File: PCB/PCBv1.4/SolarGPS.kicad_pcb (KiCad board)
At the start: 2 copper layers, 78 x 32 mm, 43 parts, among them J1 Conn_01x24_Female, J2 GND, J3 GND, J4 Conn_02x03_Odd_Even, J5 Solar2+, J6 Solar1+, J7 Screw_Terminal_01x01, J8 Conn_01x04_Male, Q1 Q_NMOS_GSD, U1 STM32L011G4Ux, U2 MAX-M10Q, U6 LIS3DH, Y1 32.768

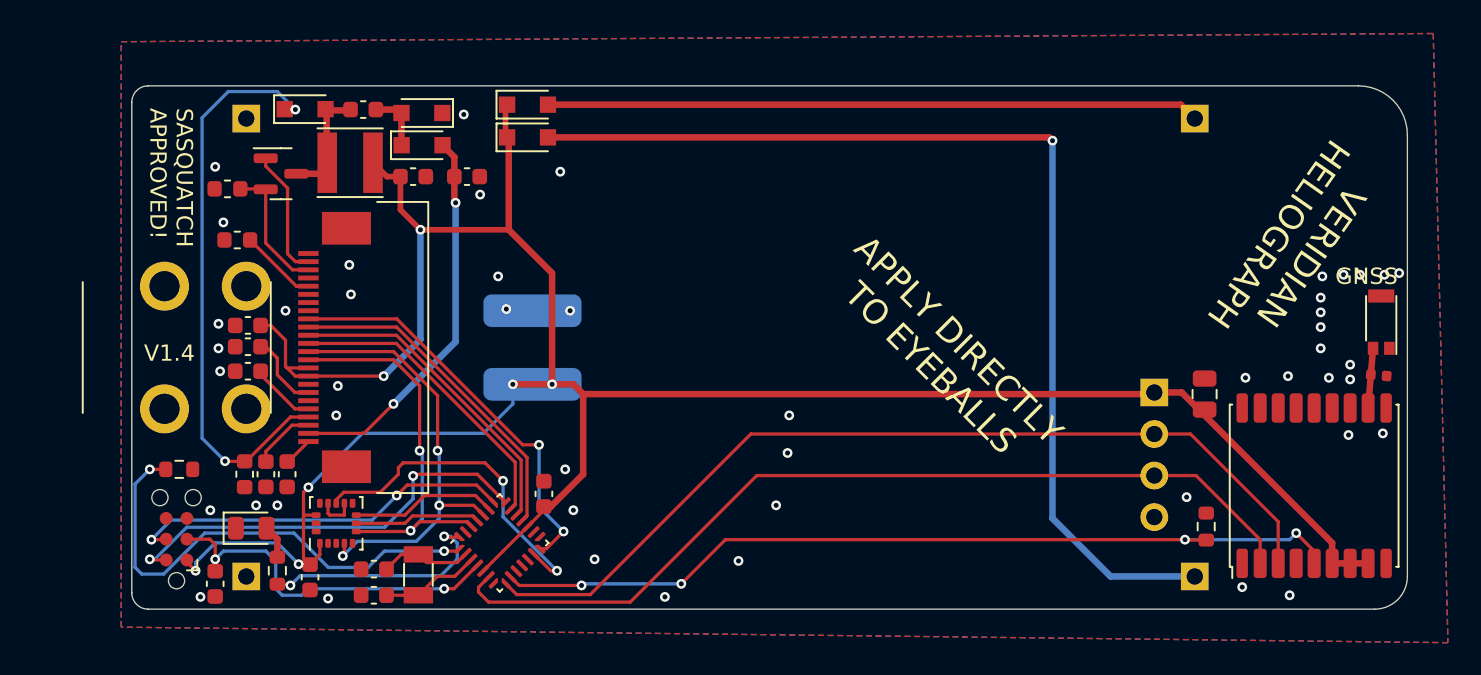
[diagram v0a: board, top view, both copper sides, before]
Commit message: firmware stuff
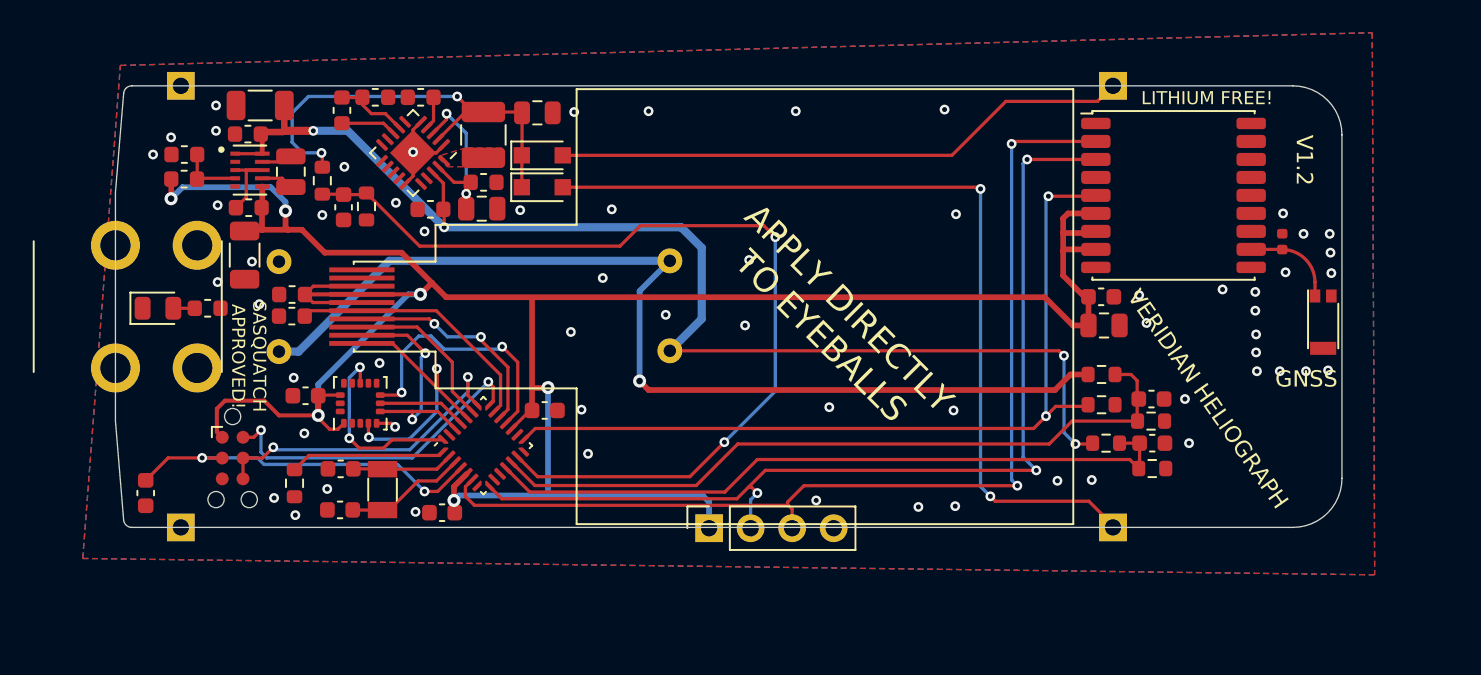
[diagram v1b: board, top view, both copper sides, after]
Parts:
- removed C22: 1uF, Capacitor_SMD:C_0603_1608Metric
- removed D4, D5, D6: B0530WS, Diode_SMD:D_SOD-323_HandSoldering
- removed L1: 47uH, Inductor_SMD:L_Taiyo-Yuden_NR-40xx
- removed Q1: Q_NMOS_GSD, Package_TO_SOT_SMD:SOT-23
- added C11: 1uF, Capacitor_SMD:C_0603_1608Metric, F.Cu at (75.2, 69.8)
- added C12: 47uF, Capacitor_SMD:C_1206_3216Metric, F.Cu at (57.9, 51.2)
- added C13: 4.7uF, Capacitor_SMD:C_0805_2012Metric, F.Cu at (109.5, 64.7)
- added C14: 10F, Veridian-Library-KiCad:SCCT20E106SRB, B.Cu at (82.9, 63.5)
- added C17: 10F, Veridian-Library-KiCad:SCCT20E106SRB, B.Cu at (59.0, 63.5)
- added C19: 10nF, Capacitor_SMD:C_0603_1608Metric, F.Cu at (71.5, 55.9)
- added C23: 10nF, Capacitor_SMD:C_0603_1608Metric, F.Cu at (112.4, 71.8)
- added C28: 10nF, Capacitor_SMD:C_0603_1608Metric, F.Cu at (63.0, 57.4)
- added L2: 0.47uH, Inductor_SMD:L_0806_2016Metric, F.Cu at (59.7, 55.2)
- added L3: 22uH, Inductor_SMD:L_1210_3225Metric, F.Cu at (71.5, 53.0)
- added R12: 1M, Resistor_SMD:R_0603_1608Metric, F.Cu at (109.6, 71.8)
- added R13: 1M, Resistor_SMD:R_0603_1608Metric, F.Cu at (112.4, 73.4)
- added R14: 1M, Resistor_SMD:R_0603_1608Metric, F.Cu at (61.6, 55.8)
- added R15: 1M, Resistor_SMD:R_0603_1608Metric, F.Cu at (64.3, 57.4)
- added R4: 432k, Resistor_SMD:R_0603_1608Metric, F.Cu at (53.2, 55.7)
- added R5: 91k, Resistor_SMD:R_0603_1608Metric, F.Cu at (53.2, 54.2)
- added R6: 1M, Resistor_SMD:R_0603_1608Metric, F.Cu at (112.3, 70.5)
- added ROV3: 4.30M, Resistor_SMD:R_0603_1608Metric, F.Cu at (64.9, 50.7)
- added ROV4: 8.66M, Resistor_SMD:R_0603_1608Metric, F.Cu at (62.9, 51.5)
- added U5: BQ25505, Package_DFN_QFN:QFN-20-1EP_3.5x3.5mm_P0.5mm_EP2x2mm, F.Cu at (67.2, 54.1)
- added U7: TPS63802, Margo_Lib:VREG_TPS63802DLAR, F.Cu at (57.2, 55.1)
- C15, C16, C18, C6: value 1uF -> 10nF
- C2, C3: value 1uF -> 4.7uF; footprint Capacitor_SMD:C_0603_1608Metric -> Capacitor_SMD:C_0805_2012Metric
- C5: value 22uF -> 10nF; footprint Capacitor_SMD:C_0805_2012Metric -> Capacitor_SMD:C_0603_1608Metric
- C7: value 1uF -> 47uF; footprint Capacitor_SMD:C_0603_1608Metric -> Capacitor_SMD:C_1206_3216Metric
- C8: value 25F -> 1uF; footprint Heliograph:TPLC3R8-25MR8X20 -> Capacitor_SMD:C_0603_1608Metric; moved to F.Cu
- D1, D3: value B0530WS -> Schottky
- J1: value Conn_01x24_Female -> Conn_01x10_Female; footprint Heliograph:ER-CON24HT-1 -> Margo_Lib:LS013B7DH03
- J2: value GND -> Solar1+
- J6: value Solar1+ -> GND
- J8: moved to F.Cu
- R1: value 1M -> 91k
- R2: value 120 -> 1M
- R3: value 2.2 -> 390
- U1: value STM32L011G4Ux -> STM32L011G3Ux
- moved J6 66.9 mm to (53.0, 77.0), turned to 0 degrees
- moved J2 60.9 mm to (110.0, 50.0), turned to 0 degrees
- moved C5 59.6 mm to (57.1, 57.5), turned to 0 degrees
- moved C16 55.3 mm to (112.3, 69.2)
- moved R2 51.8 mm to (109.3, 67.7), turned to 180 degrees
- moved C21 39.5 mm to (109.3, 62.9), turned to 0 degrees
- moved J8 28.5 mm to (85.3, 77.0), turned to 90 degrees
- moved C3 27.6 mm to (74.8, 51.6), turned to 0 degrees
- moved C8 24.6 mm to (57.1, 53.0)
- moved C2 20.1 mm to (71.4, 57.5), turned to 180 degrees
- moved C6 19.8 mm to (67.7, 50.7)
- moved U2 19.7 mm to (113.7, 56.7), turned to 0 degrees
- moved D2 14.6 mm to (51.6, 63.6)
- moved C15 13.2 mm to (68.3, 57.5)
- moved C7 11.4 mm to (56.9, 60.4), turned to 90 degrees
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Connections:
- C15 pad 2: VDD -> VBAT
- C16 pad 1: /CORE -> GND
- C16 pad 2: GND -> VBATMID_SENSE
- C2 pad 1: /VCOM -> GND
- C2 pad 2: GND -> VSTOR
- C20 pad 1: /VGH -> GND
- C20 pad 2: GND -> DISP_EN
- C21 pad 1: GND -> VDD
- C21 pad 2: /VGL -> GND
- C3 pad 1: /VSL -> SOLAR+
- C5 pad 1: VDD -> GND
- C5 pad 2: GND -> VDD
- C6 pad 1: /VSH1 -> Net-(C6-Pad1)
- C8 pad 1: VDD -> GND
- C8 pad 2: GND -> VBAT
- C9 pad 1: /VSH2 -> GND
- C9 pad 2: GND -> VDD
- D1 pad 1: VDD -> SOLAR+
- D3 pad 1: VDD -> SOLAR+
- J1 pad 1: unconnected-(J1-Pad1) -> SPI_CLK
- J1 pad 10: DISP_RES# -> GND
- J1 pad 2: /GDR -> SPI_MOSI
- J1 pad 3: /RESE -> DISP_CS
- J1 pad 4: unconnected-(J1-Pad4) -> EXTCOMIN
- J1 pad 5: /VSH2 -> DISP_EN
- J1 pad 6: unconnected-(J1-Pad6) -> VDD
- J1 pad 7: unconnected-(J1-Pad7) -> VDD
- J1 pad 8: GND -> VDD
- J1 pad 9: DISP_BUSY -> GND
- J2 pad 1: GND -> Net-(D3-Pad2)
- J4 pad 4: /SWDCLK -> SWO
- J4 pad 6: unconnected-(J4-Pad6) -> SWO
- J6 pad 1: Net-(D3-Pad2) -> GND
- R2 pad 1: Net-(D2-Pad2) -> VBATMID_SENSE
- R2 pad 2: LED -> VBATMID
- R3 pad 1: GND -> LED
- R3 pad 2: /RESE -> Net-(D2-Pad2)
- U1 pad 11: unconnected-(U1-Pad11) -> VBAT_SENSE
- U1 pad 12: unconnected-(U1-Pad12) -> VBATMID_SENSE
- U1 pad 13: LIS_INT -> SOLAR_SENSE1
- U1 pad 14: DISP_BUSY -> unconnected-(U1-Pad14)
- U1 pad 15: VBAT_OK -> GPS_EXINT
- U1 pad 18: DISP_RES# -> LIS_CS
- U1 pad 19: DISP_DC -> EXTCOMIN
- U1 pad 20: DISP_CS -> DISP_EN
- U1 pad 22: /SWDCLK -> SWO
- U1 pad 23: LIS_CS -> DISP_CS
- U1 pad 27: unconnected-(U1-Pad27) -> GND
- U1 pad 28: LED -> LIS_INT
- U1 pad 9: GPS_EXINT -> unconnected-(U1-Pad9)
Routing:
- net VBAT: track 0.00 -> 76.2 mm, vias 0 -> 4
- net VBATMID: track 0.00 -> 62.4 mm, vias 0 -> 1
- net SOLAR_SENSE1: track 0.00 -> 57.8 mm, vias 0 -> 2
- net VBATMID_SENSE: track 0.00 -> 44.5 mm
- net VBAT_SENSE: track 0.00 -> 43.2 mm
- net /VGH: track 35.3 -> 0.00 mm, vias 2 -> 0
- net SOLAR+: track 0.00 -> 27.7 mm, vias 0 -> 2
- net DISP_BUSY: track 25.1 -> 0.00 mm, vias 2 -> 0
- net /SWDCLK: track 23.7 -> 0.00 mm, vias 2 -> 0
- net /VGL: track 23.7 -> 0.00 mm, vias 2 -> 0
- net DISP_RES#: track 20.6 -> 0.00 mm
- net BOOT0: track 29.7 -> 9.54 mm, vias 2 -> 0
- net SWO: track 0.00 -> 19.7 mm, vias 0 -> 2
- net DISP_DC: track 19.6 -> 0.00 mm
- net DISP_EN: track 0.00 -> 16.1 mm
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- added copper zone on F.Cu, net Net-(L3-Pad2)
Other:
- board size 78 x 32 mm -> 75 x 27 mm
- board text added: "LITHIUM FREE!"
- board text added: "V1.2"
- board text removed: "V1.4"
- board text removed: "VDD MOSI MISO GND"
